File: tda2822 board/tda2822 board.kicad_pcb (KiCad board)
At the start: 2 copper layers, 38.6 x 27.8 mm, 14 parts, among them J1 Conn_01x02_Female, J2 Conn_01x02_Female, J3 Conn_01x02_Female, U1 TDA2822

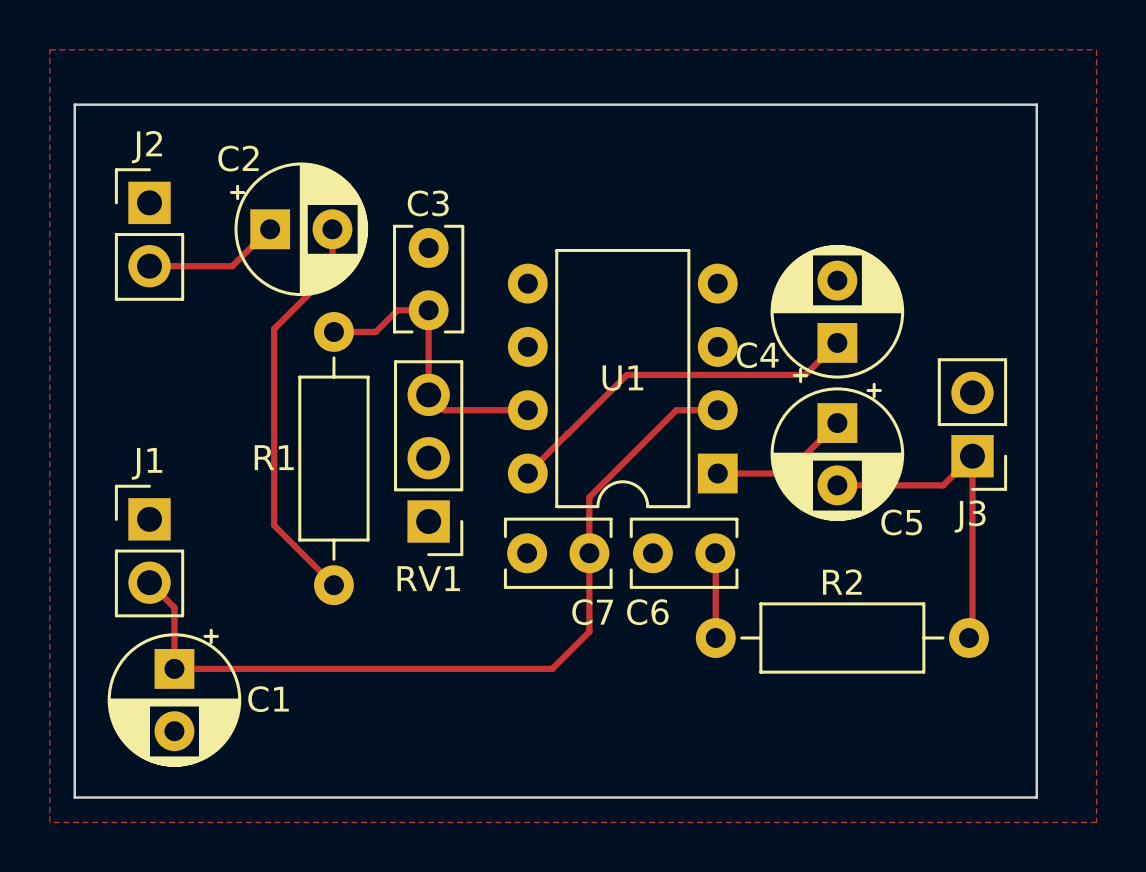
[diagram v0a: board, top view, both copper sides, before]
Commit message: Antenna mounts
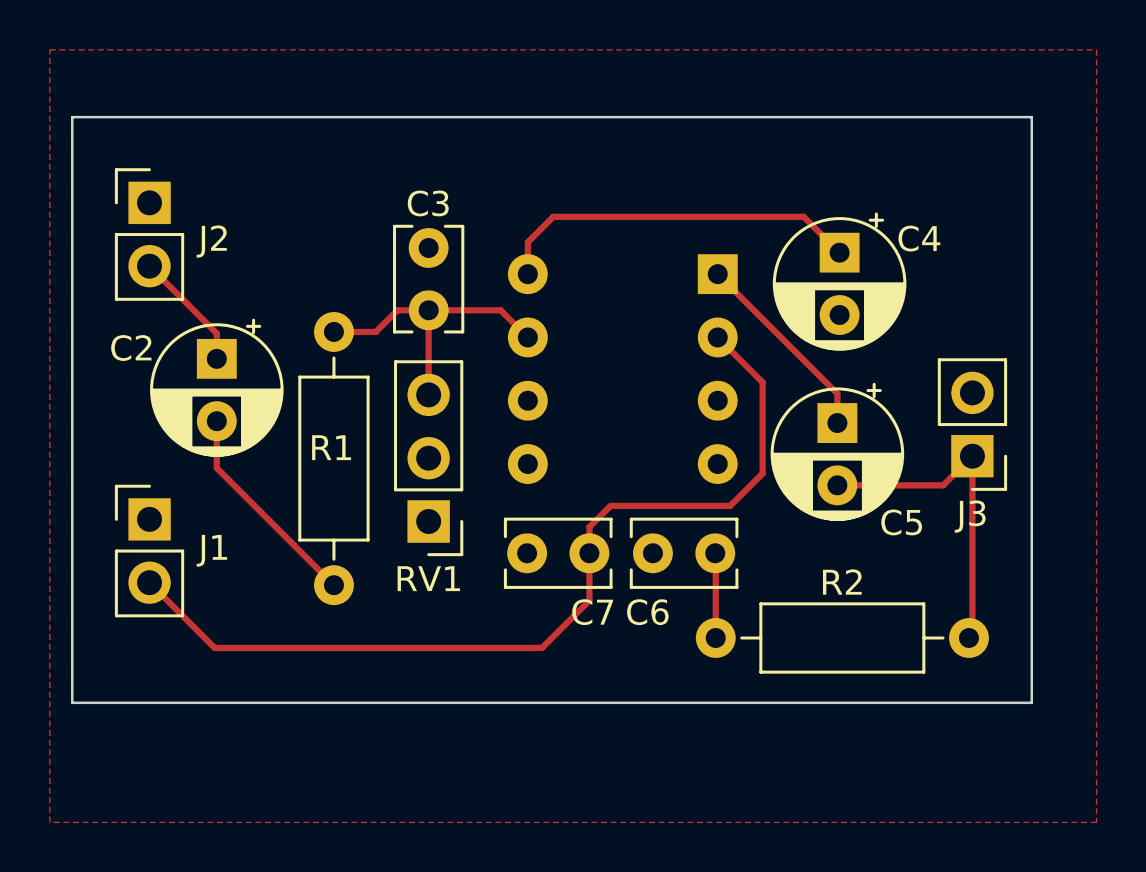
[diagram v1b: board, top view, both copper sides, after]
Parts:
- removed C1: 100u, Capacitor_THT:CP_Radial_D5.0mm_P2.50mm
- U1: moved to B.Cu
- moved U1 8.00 mm to (185.8, 85.0)
- moved C2 5.62 mm to (165.7, 88.4), turned to -90 degrees
- moved C4 3.62 mm to (190.7, 84.1), turned to -90 degrees
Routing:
- net Net-(C2-Pad2): track 16.2 -> 8.53 mm
- net +5V: track 33.1 -> 36.5 mm
- net Net-(C5-Pad1): track 5.64 -> 7.96 mm
- net Net-(C2-Pad1): track 5.45 -> 4.84 mm
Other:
- board size 38.6 x 27.8 mm -> 38.5 x 23.5 mm
